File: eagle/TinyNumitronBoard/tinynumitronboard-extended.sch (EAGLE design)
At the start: 51 parts

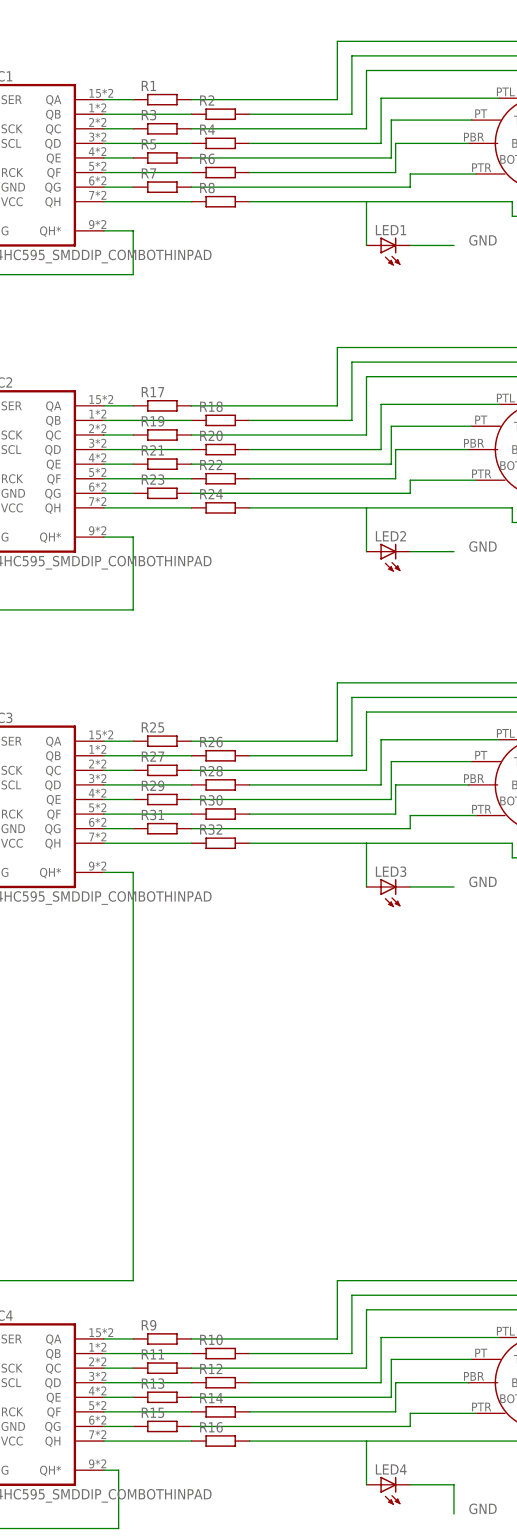
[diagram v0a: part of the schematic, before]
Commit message: Version 1.0 sent to production with nice image on the top.
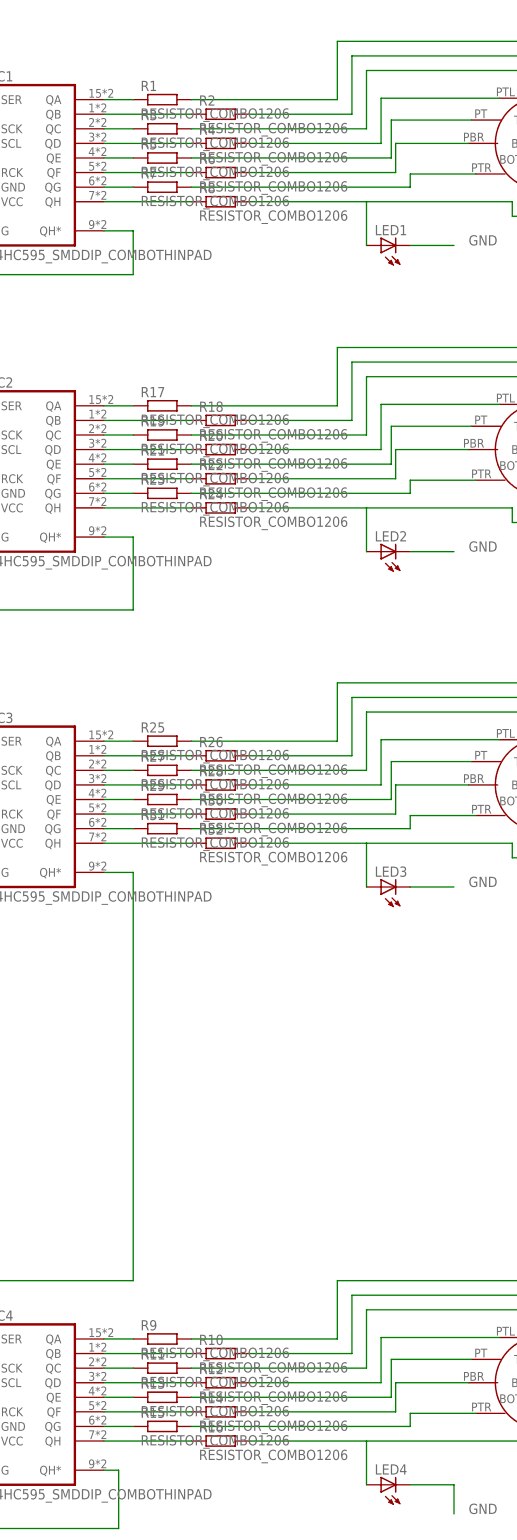
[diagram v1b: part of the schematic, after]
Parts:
- R1, R10, R11, R12, R13, R14, R15, R16, R17, R18, R19, R2, R20, R21, R22, R23, R24, R25, R26, R27, R28, R29, R3, R30, R31, R32, R4, R5, R6, R7, R8, R9: value (none) -> RESISTOR_COMBO1206; device resistor:R-EU_0207/10 -> kalshagar:RESISTOR_COMBO1206
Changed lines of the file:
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@@
 <parts>
 <part name="U$1" library="kalshagar" deviceset="IV16TINY_NUMITRON" device=""/>
-<part name="R1" library="resistor" deviceset="R-EU_" device="0207/10"/>
-<part name="R2" library="resistor" deviceset="R-EU_" device="0207/10"/>
-<part name="R3" library="resistor" deviceset="R-EU_" device="0207/10"/>
-<part name="R4" library="resistor" deviceset="R-EU_" device="0207/10"/>
-<part name="R5" library="resistor" deviceset="R-EU_" device="0207/10"/>
-<part name="R6" library="resistor" deviceset="R-EU_" device="0207/10"/>
-<part name="R7" library="resistor" deviceset="R-EU_" device="0207/10"/>
+<part name="R1" library="kalshagar" deviceset="RESISTOR_COMBO1206" device=""/>
+<part name="R2" library="kalshagar" deviceset="RESISTOR_COMBO1206" device=""/>
+<part name="R3" library="kalshagar" deviceset="RESISTOR_COMBO1206" device=""/>
+<part name="R4" library="kalshagar" deviceset="RESISTOR_COMBO1206" device=""/>
+<part name="R5" library="kalshagar" deviceset="RESISTOR_COMBO1206" device=""/>
+<part name="R6" library="kalshagar" deviceset="RESISTOR_COMBO1206" device=""/>
+<part name="R7" library="kalshagar" deviceset="RESISTOR_COMBO1206" device=""/>
 <part name="JP_INPUT" library="SparkFun" deviceset="M06" device="SIP"/>
 <part name="LED1" library="led" deviceset="LED" device="KA-3528ASYC"/>
-<part name="R8" library="resistor" deviceset="R-EU_" device="0207/10"/>
+<part name="R8" library="kalshagar" deviceset="RESISTOR_COMBO1206" device=""/>
 <part name="C1" library="resistor" deviceset="C-EU" device="050-024X044" value="1uF"/>
 <part name="JP_OUTPUT" library="SparkFun" deviceset="M06" device="SIP"/>
 <part name="U$2" library="kalshagar" deviceset="IV16TINY_NUMITRON" device=""/>
-<part name="R9" library="resistor" deviceset="R-EU_" device="0207/10"/>
-<part name="R10" library="resistor" deviceset="R-EU_" device="0207/10"/>
-<part name="R11" library="resistor" deviceset="R-EU_" device="0207/10"/>
-<part name="R12" library="resistor" deviceset="R-EU_" device="0207/10"/>
-<part name="R13" library="resistor" deviceset="R-EU_" device="0207/10"/>
-<part name="R14" library="resistor" deviceset="R-EU_" device="0207/10"/>
-<part name="R15" library="resistor" deviceset="R-EU_" device="0207/10"/>
+<part name="R9" library="kalshagar" deviceset="RESISTOR_COMBO1206" device=""/>
+<part name="R10" library="kalshagar" deviceset="RESISTOR_COMBO1206" device=""/>
+<part name="R11" library="kalshagar" deviceset="RESISTOR_COMBO1206" device=""/>
+<part name="R12" library="kalshagar" deviceset="RESISTOR_COMBO1206" device=""/>
+<part name="R13" library="kalshagar" deviceset="RESISTOR_COMBO1206" device=""/>
+<part name="R14" library="kalshagar" deviceset="RESISTOR_COMBO1206" device=""/>
+<part name="R15" library="kalshagar" deviceset="RESISTOR_COMBO1206" device=""/>
 <part name="LED4" library="led" deviceset="LED" device="KA-3528ASYC"/>
-<part name="R16" library="resistor" deviceset="R-EU_" device="0207/10"/>
+<part name="R16" library="kalshagar" deviceset="RESISTOR_COMBO1206" device=""/>
 <part name="UC1" library="kalshagar" deviceset="74HC595_SMDDIP_COMBO" device="THINPAD"/>
 <part name="UC4" library="kalshagar" deviceset="74HC595_SMDDIP_COMBO" device="THINPAD"/>
 <part name="U$5" library="kalshagar" deviceset="IV16TINY_NUMITRON" device=""/>
-<part name="R17" library="resistor" deviceset="R-EU_" device="0207/10"/>
-<part name="R18" library="resistor" deviceset="R-EU_" device="0207/10"/>
-<part name="R19" library="resistor" deviceset="R-EU_" device="0207/10"/>
-<part name="R20" library="resistor" deviceset="R-EU_" device="0207/10"/>
-<part name="R21" library="resistor" deviceset="R-EU_" device="0207/10"/>
-<part name="R22" library="resistor" deviceset="R-EU_" device="0207/10"/>
-<part name="R23" library="resistor" deviceset="R-EU_" device="0207/10"/>
+<part name="R17" library="kalshagar" deviceset="RESISTOR_COMBO1206" device=""/>
+<part name="R18" library="kalshagar" deviceset="RESISTOR_COMBO1206" device=""/>
+<part name="R19" library="kalshagar" deviceset="RESISTOR_COMBO1206" device=""/>
+<part name="R20" library="kalshagar" deviceset="RESISTOR_COMBO1206" device=""/>
+<part name="R21" library="kalshagar" deviceset="RESISTOR_COMBO1206" device=""/>
+<part name="R22" library="kalshagar" deviceset="RESISTOR_COMBO1206" device=""/>
+<part name="R23" library="kalshagar" deviceset="RESISTOR_COMBO1206" device=""/>
 <part name="LED2" library="led" deviceset="LED" device="KA-3528ASYC"/>
-<part name="R24" library="resistor" deviceset="R-EU_" device="0207/10"/>
+<part name="R24" library="kalshagar" deviceset="RESISTOR_COMBO1206" device=""/>
 <part name="UC2" library="kalshagar" deviceset="74HC595_SMDDIP_COMBO" device="THINPAD"/>
 <part name="U$7" library="kalshagar" deviceset="IV16TINY_NUMITRON" device=""/>
-<part name="R25" library="resistor" deviceset="R-EU_" device="0207/10"/>
-<part name="R26" library="resistor" deviceset="R-EU_" device="0207/10"/>
-<part name="R27" library="resistor" deviceset="R-EU_" device="0207/10"/>
-<part name="R28" library="resistor" deviceset="R-EU_" device="0207/10"/>
-<part name="R29" library="resistor" deviceset="R-EU_" device="0207/10"/>
-<part name="R30" library="resistor" deviceset="R-EU_" device="0207/10"/>
-<part name="R31" library="resistor" deviceset="R-EU_" device="0207/10"/>
+<part name="R25" library="kalshagar" deviceset="RESISTOR_COMBO1206" device=""/>
+<part name="R26" library="kalshagar" deviceset="RESISTOR_COMBO1206" device=""/>
+<part name="R27" library="kalshagar" deviceset="RESISTOR_COMBO1206" device=""/>
+<part name="R28" library="kalshagar" deviceset="RESISTOR_COMBO1206" device=""/>
+<part name="R29" library="kalshagar" deviceset="RESISTOR_COMBO1206" device=""/>
+<part name="R30" library="kalshagar" deviceset="RESISTOR_COMBO1206" device=""/>
+<part name="R31" library="kalshagar" deviceset="RESISTOR_COMBO1206" device=""/>
 <part name="LED3" library="led" deviceset="LED" device="KA-3528ASYC"/>
-<part name="R32" library="resistor" deviceset="R-EU_" device="0207/10"/>
+<part name="R32" library="kalshagar" deviceset="RESISTOR_COMBO1206" device=""/>
 <part name="UC3" library="kalshagar" deviceset="74HC595_SMDDIP_COMBO" device="THINPAD"/>
 <part name="H4" library="holes" deviceset="MOUNT-HOLE" device="2.8"/>
